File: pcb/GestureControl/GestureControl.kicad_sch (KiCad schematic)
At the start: 77 parts, among them J1 Conn_01x04_I2I-LCD, J2 BATT, J24 Conn_02x19_Odd_Even, J25 Conn_02x19_Odd_Even, SW1 SW1, SW2 SW2, U1 AP5100_3.3, U2 AP5100_3.3

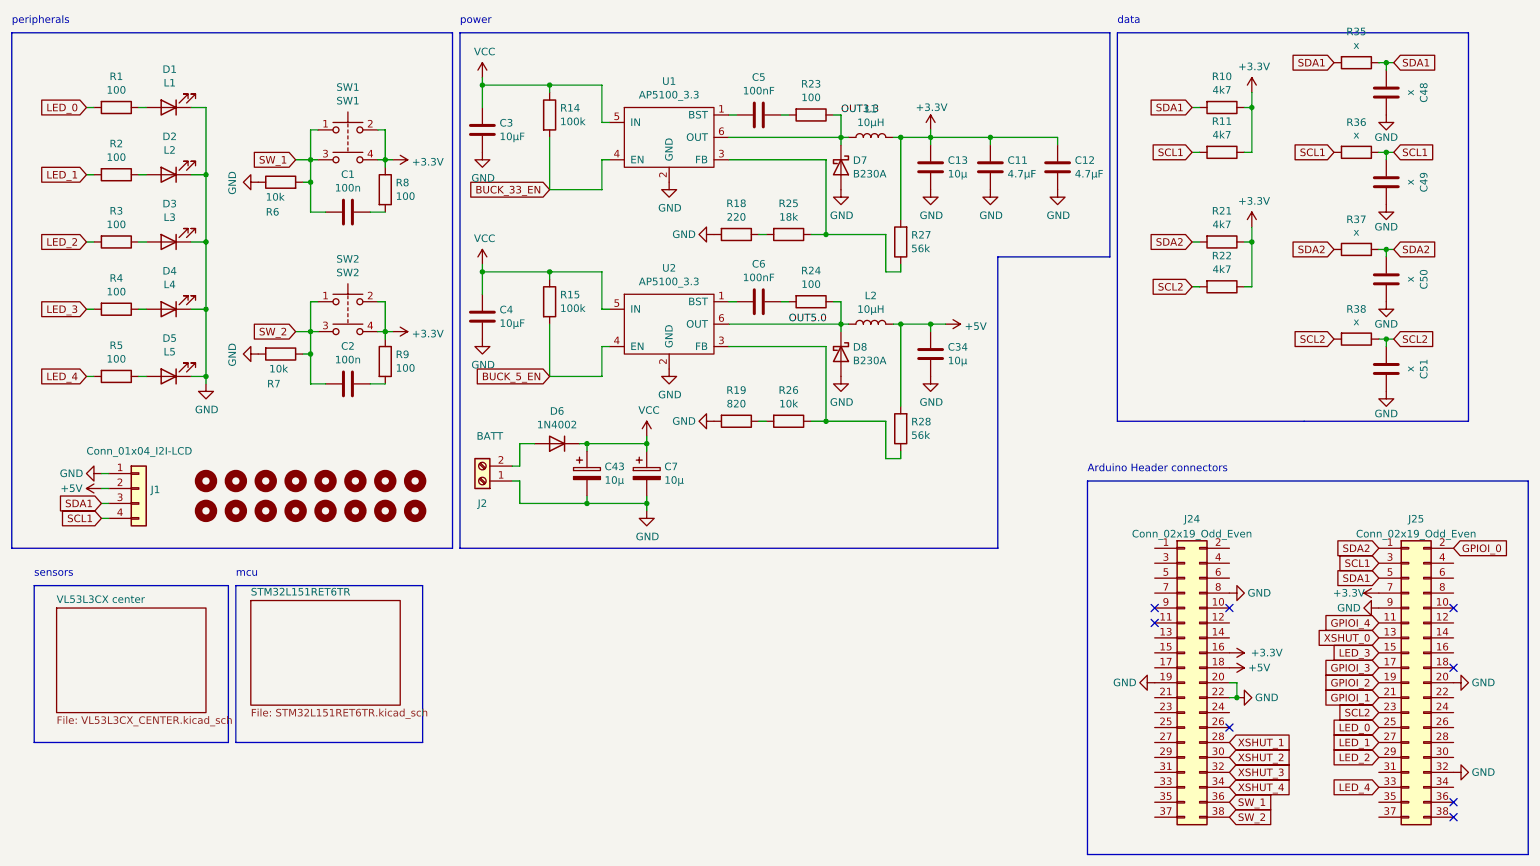
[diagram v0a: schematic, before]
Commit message: edit schematic
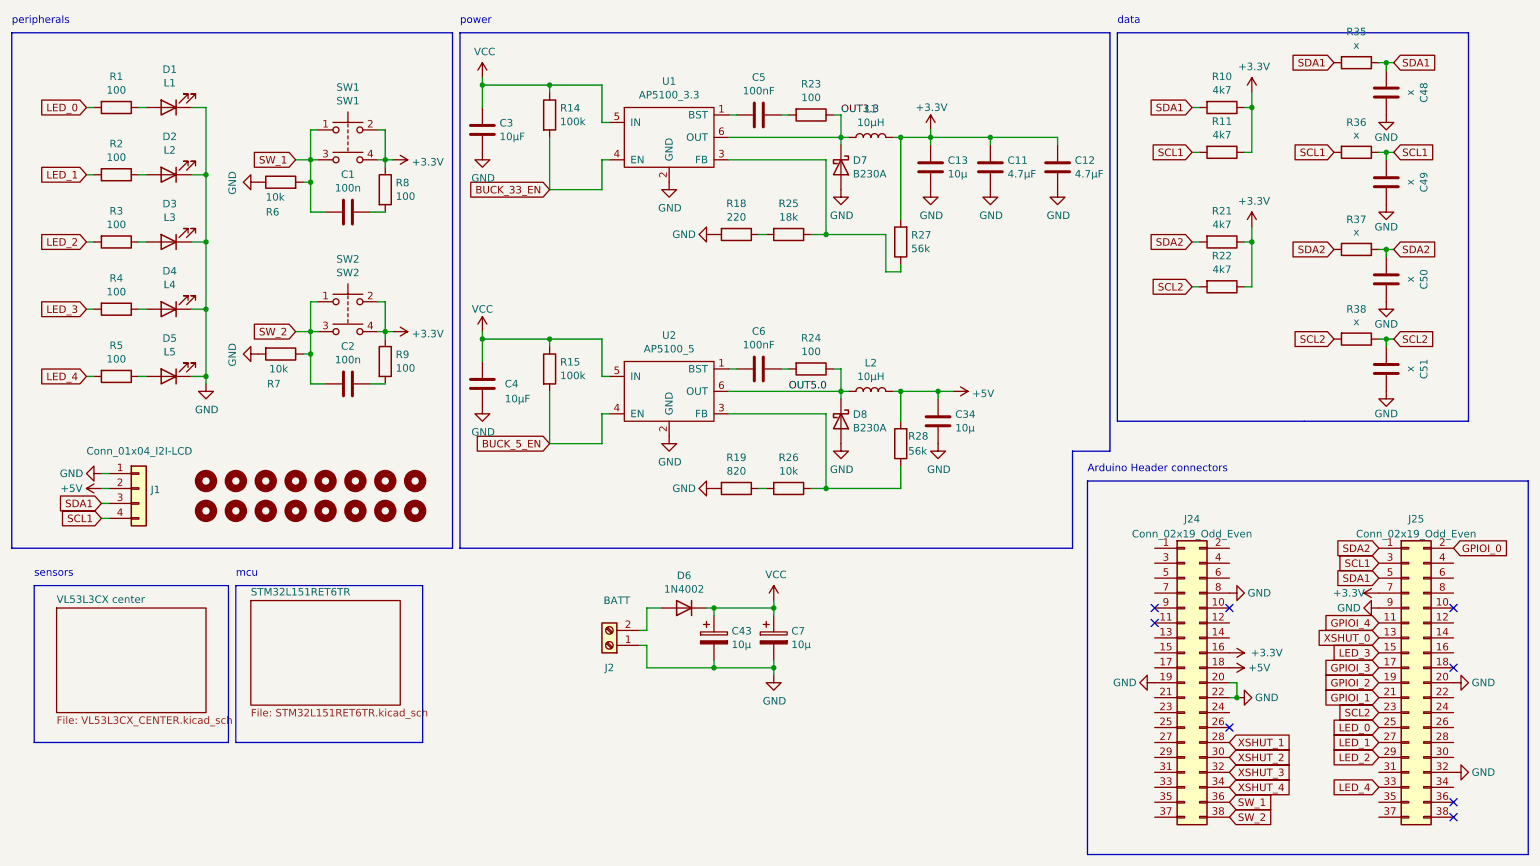
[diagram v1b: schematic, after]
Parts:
- U2: value AP5100_3.3 -> AP5100_5
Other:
- moved on the sheet: C34, C4, C43, C6, C7, D6, D8, J2, L2, R15, R19, R24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
